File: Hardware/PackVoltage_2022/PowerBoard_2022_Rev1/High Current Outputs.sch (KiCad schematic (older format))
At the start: 20 parts

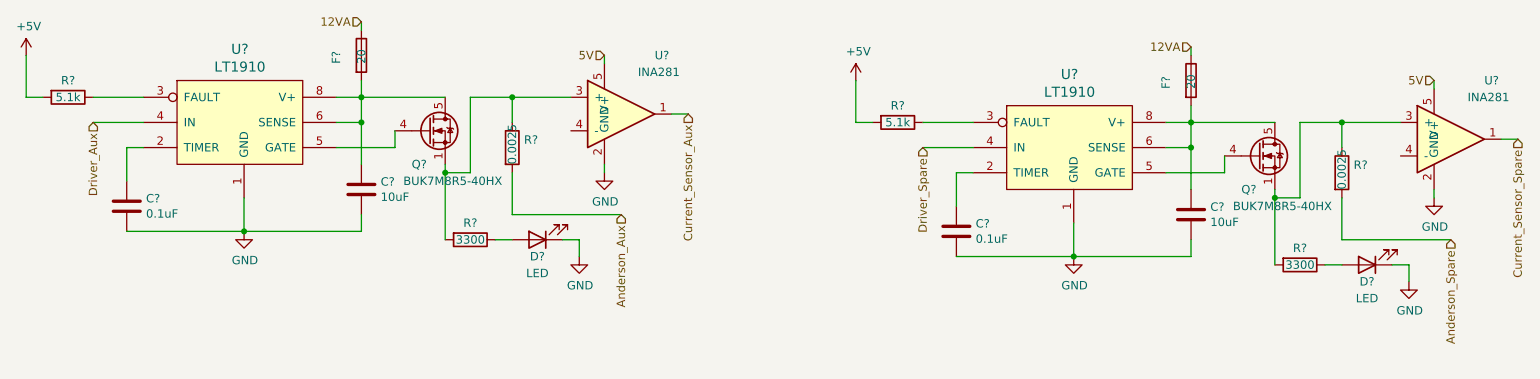
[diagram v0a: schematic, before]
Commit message: Fixed some stuff
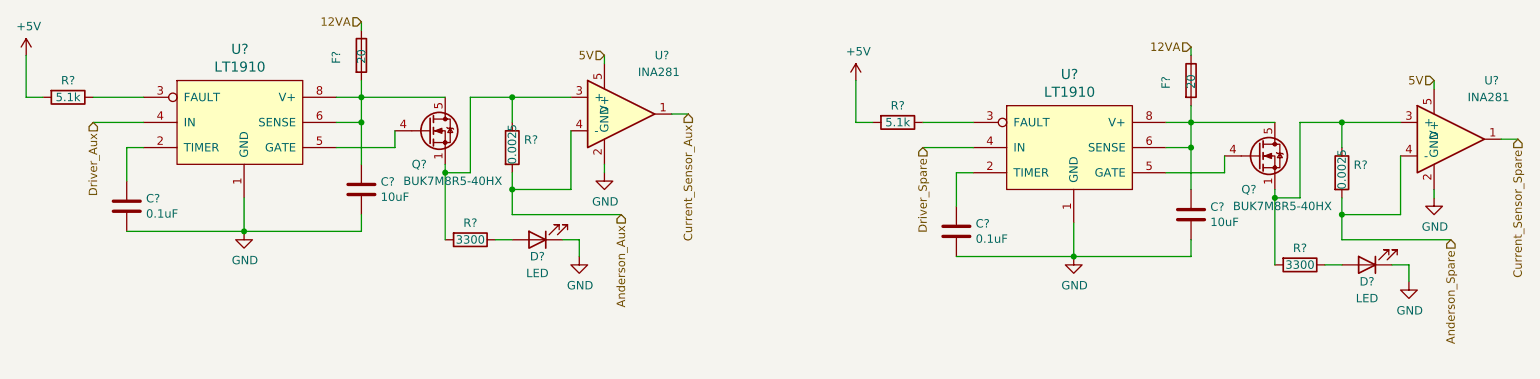
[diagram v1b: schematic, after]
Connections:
- net Anderson_Aux: now also U?.4 (-)
- net Anderson_Spare: now also U?.4 (-)
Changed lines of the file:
@@
 $Descr A4 11693 8268
 encoding utf-8
-Sheet 8 9
+Sheet 7 9
 Title ""
 Date ""
@@
 	3750 2450 4400 2450
 Wire Wire Line
-	3750 2200 3750 2450
+	3750 2200 3750 2300
 Wire Wire Line
 	3350 2150 3350 2200
@@
 	8700 2600 9350 2600
 Wire Wire Line
-	8700 2350 8700 2600
+	8700 2350 8700 2450
 Wire Wire Line
 	8300 2300 8300 2350
@@
 Wire Wire Line
 	7800 1500 7800 1450
+Wire Wire Line
+	4100 1950 4100 2300
+Wire Wire Line
+	4100 2300 3750 2300
+Connection ~ 3750 2300
+Wire Wire Line
+	3750 2300 3750 2450
+Wire Wire Line
+	9050 2100 9050 2450
+Wire Wire Line
+	9050 2450 8700 2450
+Connection ~ 8700 2450
+Wire Wire Line
+	8700 2450 8700 2600
 $EndSCHEMATC
